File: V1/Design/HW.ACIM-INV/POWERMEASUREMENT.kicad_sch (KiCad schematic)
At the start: 47 parts, among them U17 ISO OPAMP 1-CH, U18 OP-1CH, U19 OP-1CH, U6 ISEN 50mV/V, U7 ISO OPAMP 1-CH, U8 OP-1CH

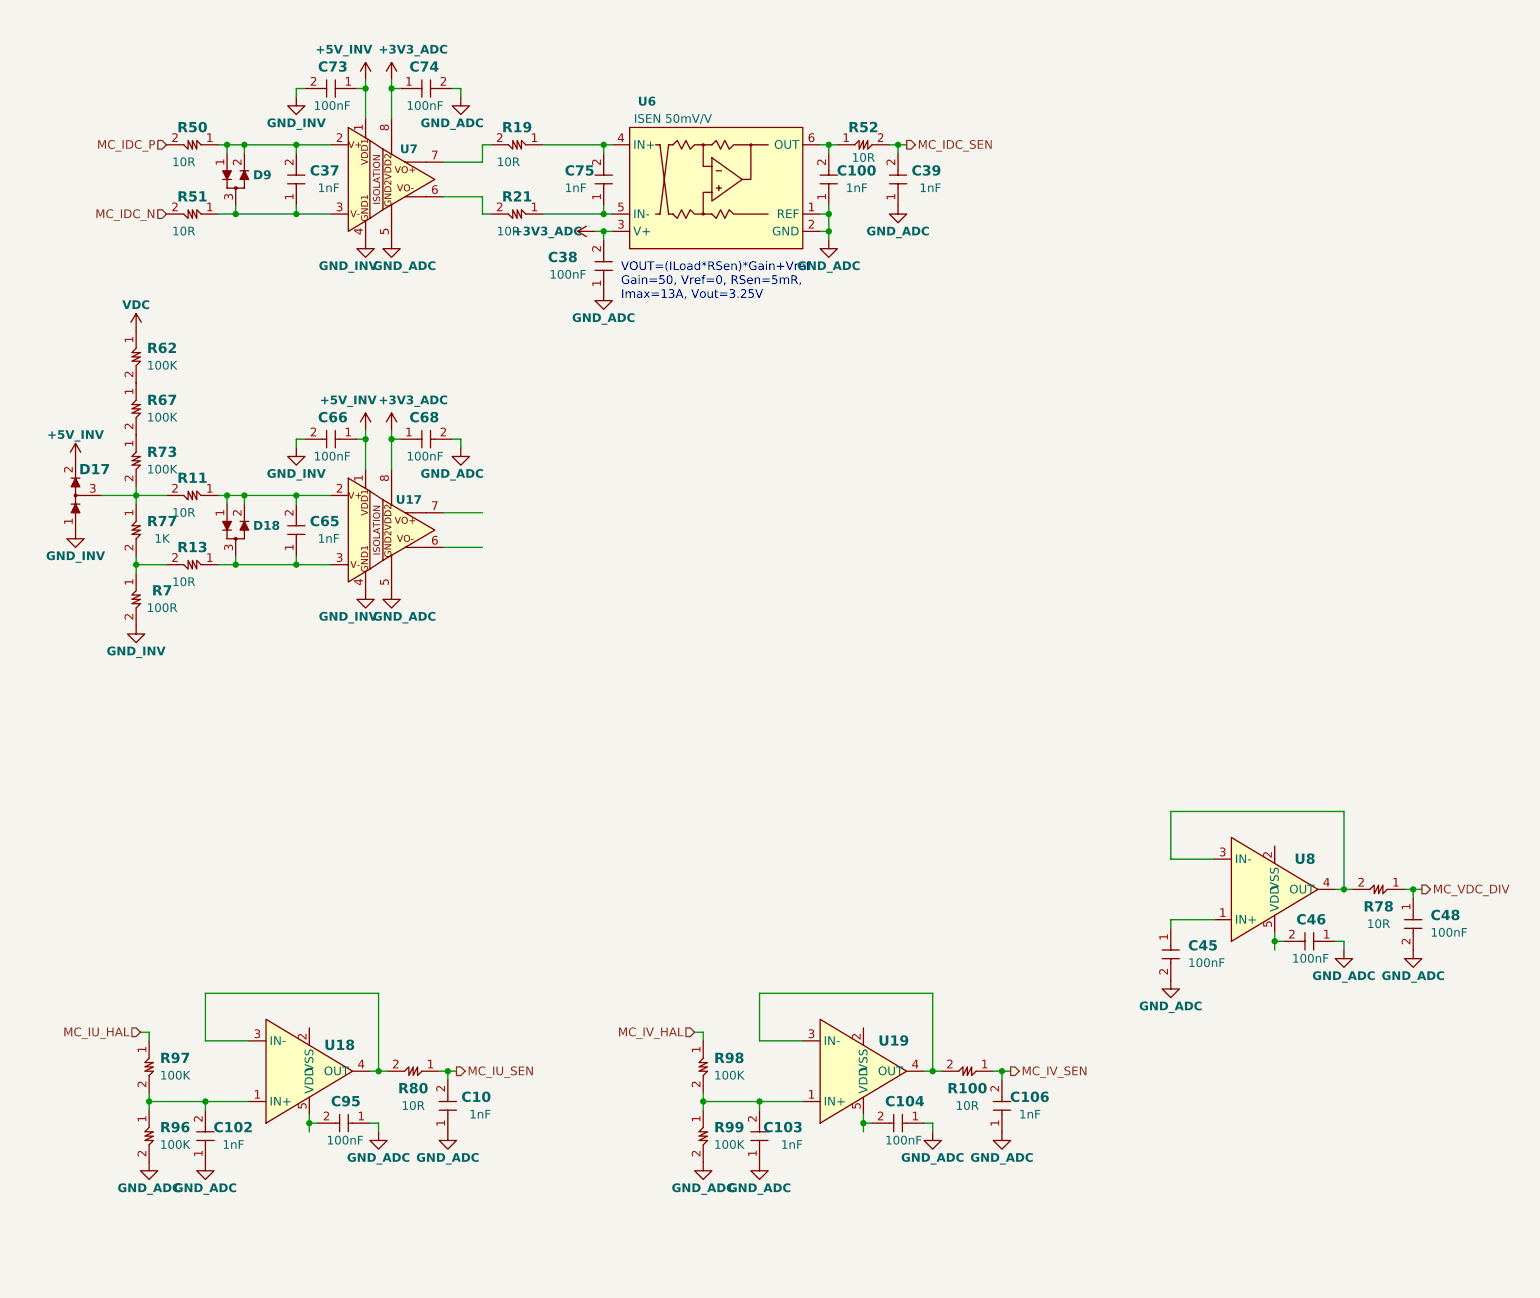
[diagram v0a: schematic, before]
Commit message: V1 schematic update 15
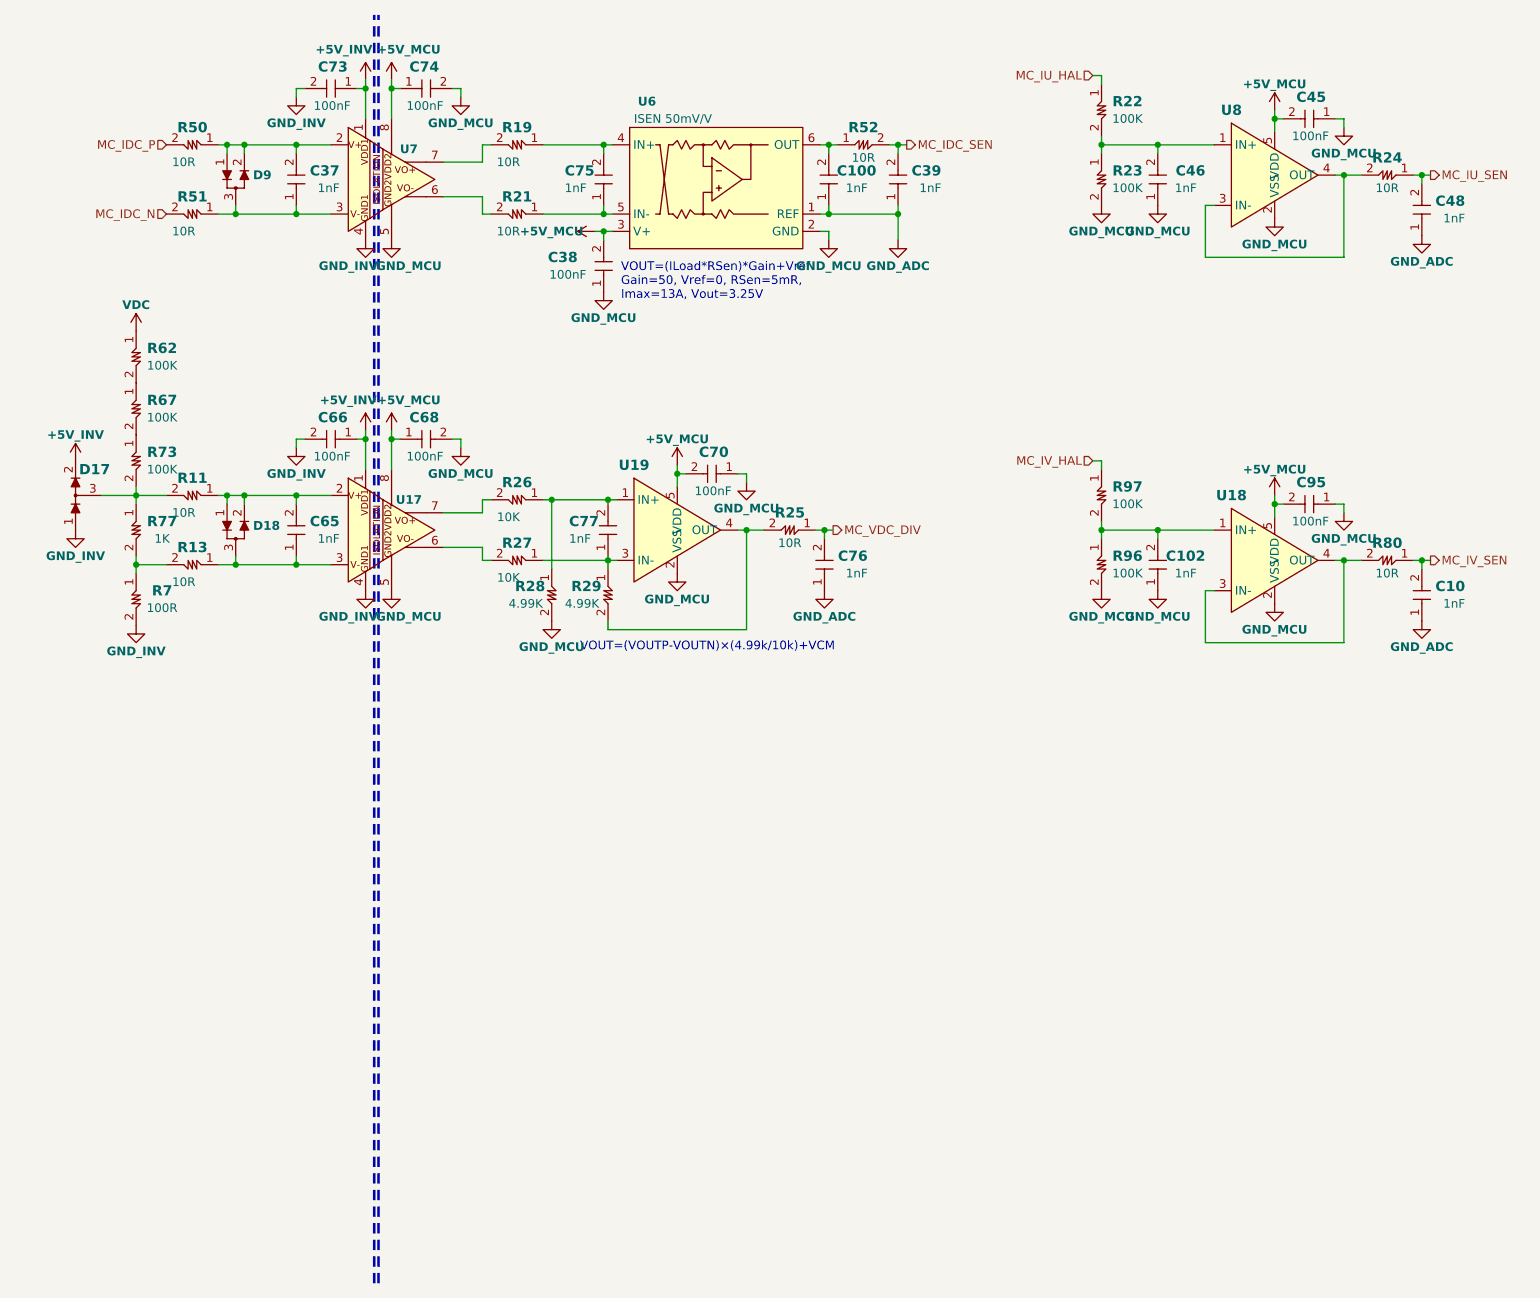
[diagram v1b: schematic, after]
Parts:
- removed C103, C106: 1nF, SAMPI:CAP0603, symbol SAMPI:CERCAP
- removed C104: 100nF, SAMPI:CAP0603, symbol SAMPI:CERCAP
- removed R100, R78: 10R, SAMPI:RES0603, symbol SAMPI:RES
- removed R98, R99: 100K, SAMPI:RES0603, symbol SAMPI:RES
- added C70: 100nF, SAMPI:CAP0603, symbol SAMPI:CERCAP
- added C76, C77: 1nF, SAMPI:CAP0603, symbol SAMPI:CERCAP
- added R22, R23: 100K, SAMPI:RES0603, symbol SAMPI:RES
- added R24, R25: 10R, SAMPI:RES0603, symbol SAMPI:RES
- added R26, R27: 10K, SAMPI:RES0603, symbol SAMPI:RES
- added R28, R29: 4.99K, SAMPI:RES0603, symbol SAMPI:RES
- C46, C48: value 100nF -> 1nF; MNP CL10B104KB8NNNC -> CL10B102KB8NNNC
- U6: MFT Diodes -> Onsemi; MNP ZXCT199QA1DW-7 -> NCS199A1RSQT2G
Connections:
- net +3V3_ADC is gone; now on net +5V_MCU: C38.2, C68.1, C74.1, U17.8 (VDD2), U6.3 (V+), U7.8 (VDD2)
- net GND_ADC: now also C48.1, C76.1; no longer C102.1, C38.1, C45.2, C46.1, C48.2, C68.2, C74.2, C95.1, R96.2, U17.5 (GND2), U6.2 (GND), U7.5 (GND2)
- net MC_IU_HAL: now also R22.1; no longer R97.1
- net MC_IU_SEN: now also C48.2, R24.1; no longer C10.2, R80.1
- net MC_IV_HAL: now also R97.1
- net MC_IV_SEN: now also C10.2, R80.1
- net MC_VDC_DIV: now also C76.2, R25.1; no longer C48.1
- net +5V_MCU: now reaches U19.5 (VDD)
- net +5V_MCU: now also C45.2, C95.2, U18.5 (VDD), U8.5 (VDD), C70.2
- net at U19.3 (IN-): now also C77.1, R27.1, R29.1; no longer U19.4 (OUT)
- net at U8.1 (IN+): now also C46.2, R22.2, R23.1; no longer C45.1
- net GND_MCU: now reaches U8.2 (VSS)
- net GND_MCU: now also C102.1, C38.1, C45.1, C46.1, C68.2, C74.2, C95.1, R96.2, U17.5 (GND2), U18.2 (VSS), U19.2 (VSS), U6.2 (GND), U7.5 (GND2), C70.1, R23.2, R28.2
- net at U8.3 (IN-), U8.4 (OUT): now also R24.2
- net at U17.6 (VOUT-): now also R27.2
- net at U17.7 (VOUT+): now also R26.2
- net at U19.1 (IN+): now also C77.2, R26.1, R28.1
- new net: R25.2, R29.2, U19.4 (OUT)
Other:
- note added: "VOUT=(VOUTP-VOUTN)×(4.99k/10k)+VCM"
- company: TON DUC THANG UNIVERSITY -> (none)
- moved on the sheet: C10, C102, C95, R80, R96, R97, U18

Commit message: V1 schematic update 16
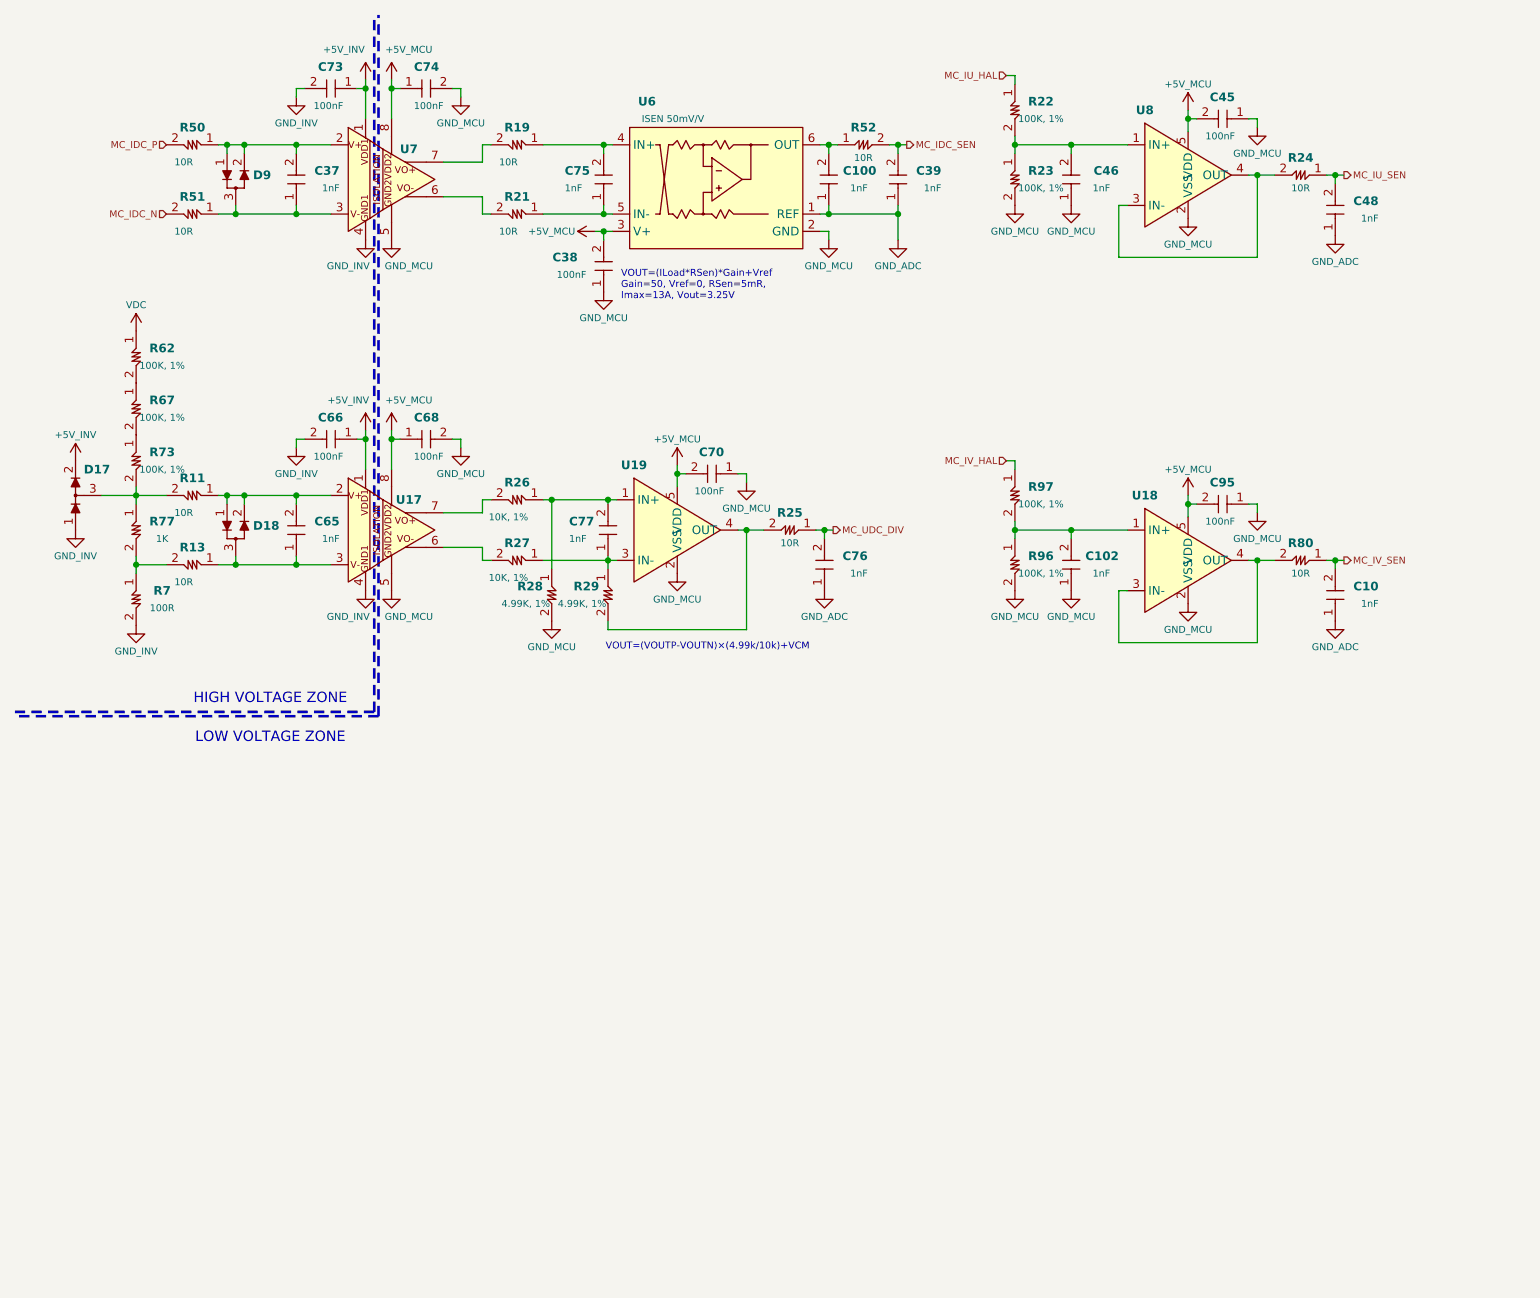
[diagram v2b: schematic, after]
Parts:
- R22, R23, R62, R67, R73, R96, R97: value 100K -> 100K, 1%
- R26, R27: value 10K -> 10K, 1%; MNP RC0603FR-0710RL -> RC0603FR-0710KL
- R28, R29: value 4.99K -> 4.99K, 1%; MFT YAGEO -> (none); MNP RC0603FR-0710RL -> (none)
- R7, R77: MFT YAGEO -> (none); MNP AC0603FR-071K1L -> (none)
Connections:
- net MC_VDC_DIV renamed MC_UDC_DIV
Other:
- note added: "HIGH VOLTAGE ZONE"
- note added: "LOW VOLTAGE ZONE"
- moved on the sheet: C10, C102, C45, C46, C48, C95, R22, R23, R24, R80, R96, R97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
